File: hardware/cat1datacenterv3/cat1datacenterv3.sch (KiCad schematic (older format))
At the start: 67 parts, among them J1 CAT1UART, J2 USB_C_Receptacle_USB2.0, J3 SPK, J4 IIC, J5 UART1, J6 UART3, J7 SPI, J8 Conn_02x02_Counter_Clockwise, J9 HLK_TTL, U1 Air724, U2 ETA8113, U3 AMS1117-3.3, U4 HLK_7628N

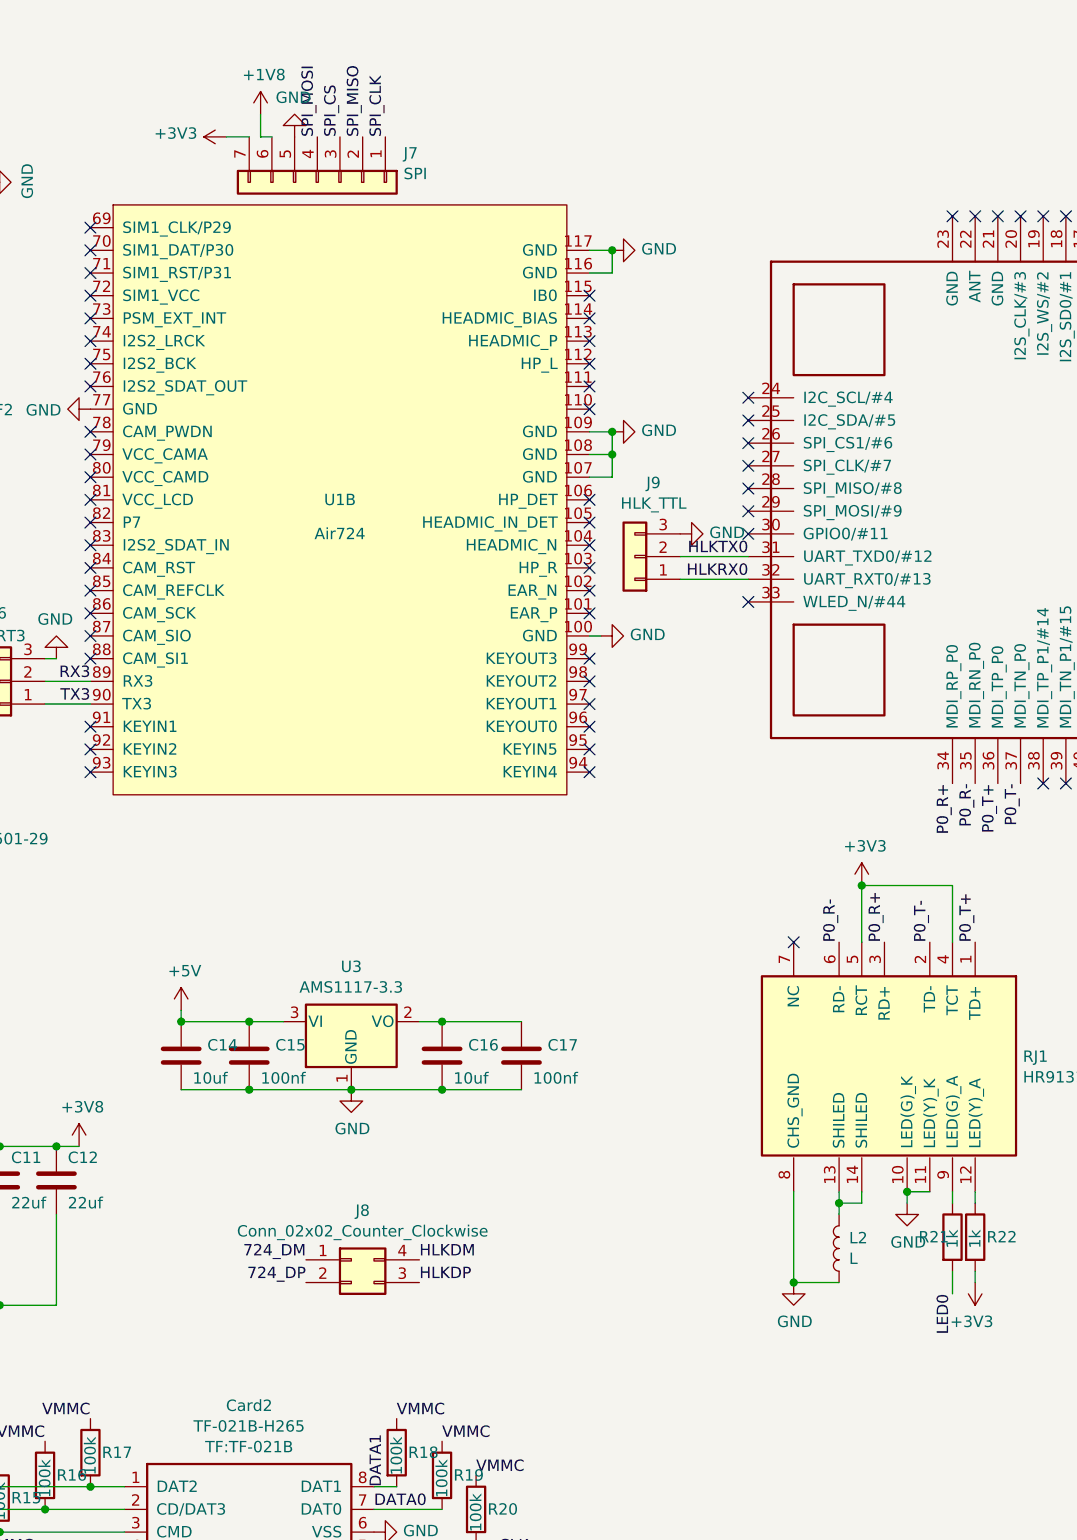
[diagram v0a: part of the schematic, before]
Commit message: add: sim加个srv05
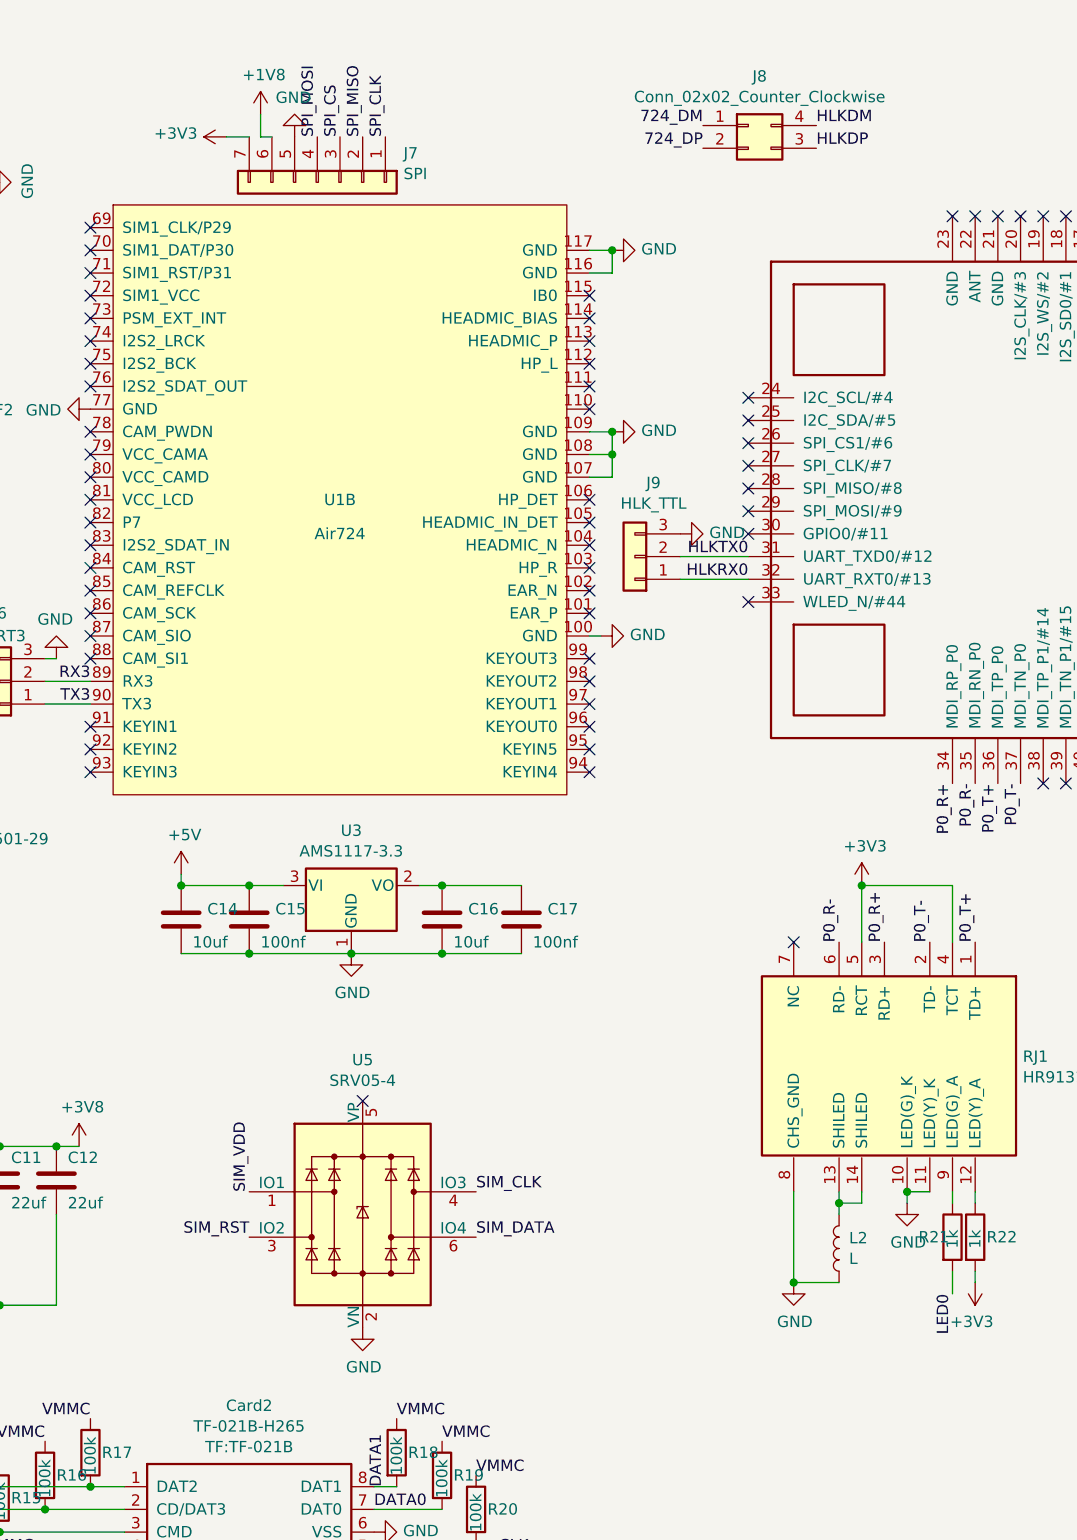
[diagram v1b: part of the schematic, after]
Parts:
- added U5: SRV05-4, Package_TO_SOT_SMD:SOT-23-6, symbol Power_Protection:SRV05-4
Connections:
- net GND: now also U5.2 (VN)
- net SIM_CLK: now also U5.4 (IO3)
- net SIM_DATA: now also U5.6 (IO4)
- net SIM_RST: now also U5.3 (IO2)
- net SIM_VDD: now also U5.1 (IO1)
- no-connect marks 97 -> 98
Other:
- moved on the sheet: C14, C15, C16, C17, J8, U3
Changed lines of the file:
@@
 L Regulator_Linear:AMS1117-3.3 U3
 U 1 1 60BE7D12
-P 6100 4850
-F 0 "U3" H 6100 5092 50  0000 C CNN
-F 1 "AMS1117-3.3" H 6100 5001 50  0000 C CNN
-F 2 "Package_TO_SOT_SMD:SOT-89-3_Handsoldering" H 6100 5050 50  0001 C CNN
-F 3 "http://www.advanced-monolithic.com/pdf/ds1117.pdf" H 6200 4600 50  0001 C CNN
-	1    6100 4850
+P 6100 4250
+F 0 "U3" H 6100 4492 50  0000 C CNN
+F 1 "AMS1117-3.3" H 6100 4401 50  0000 C CNN
+F 2 "Package_TO_SOT_SMD:SOT-89-3_Handsoldering" H 6100 4450 50  0001 C CNN
+F 3 "http://www.advanced-monolithic.com/pdf/ds1117.pdf" H 6200 4000 50  0001 C CNN
+	1    6100 4250
 	1    0    0    -1
 $EndComp
@@
 L Device:C C16
 U 1 1 60C07B48
-P 6500 5000
-F 0 "C16" H 6615 5046 50  0000 L CNN
-F 1 "10uf" H 6550 4900 50  0000 L CNN
-F 2 "Capacitor_SMD:C_0603_1608Metric_Pad1.05x0.95mm_HandSolder" H 6538 4850 50  0001 C CNN
-F 3 "~" H 6500 5000 50  0001 C CNN
-	1    6500 5000
+P 6500 4400
+F 0 "C16" H 6615 4446 50  0000 L CNN
+F 1 "10uf" H 6550 4300 50  0000 L CNN
+F 2 "Capacitor_SMD:C_0603_1608Metric_Pad1.05x0.95mm_HandSolder" H 6538 4250 50  0001 C CNN
+F 3 "~" H 6500 4400 50  0001 C CNN
+	1    6500 4400
 	1    0    0    -1
 $EndComp
@@
 L Device:C C17
 U 1 1 60C088A8
-P 6850 5000
-F 0 "C17" H 6965 5046 50  0000 L CNN
-F 1 "100nf" H 6900 4900 50  0000 L CNN
-F 2 "Capacitor_SMD:C_0603_1608Metric_Pad1.05x0.95mm_HandSolder" H 6888 4850 50  0001 C CNN
-F 3 "~" H 6850 5000 50  0001 C CNN
-	1    6850 5000
-	1    0    0    -1
-$EndComp
-Wire Wire Line
-	6400 4850 6500 4850
-Connection ~ 6500 4850
-Wire Wire Line
-	6500 4850 6850 4850
-Wire Wire Line
-	6100 5150 6500 5150
-Connection ~ 6500 5150
-Wire Wire Line
-	6500 5150 6850 5150
+P 6850 4400
+F 0 "C17" H 6965 4446 50  0000 L CNN
+F 1 "100nf" H 6900 4300 50  0000 L CNN
+F 2 "Capacitor_SMD:C_0603_1608Metric_Pad1.05x0.95mm_HandSolder" H 6888 4250 50  0001 C CNN
+F 3 "~" H 6850 4400 50  0001 C CNN
+	1    6850 4400
+	1    0    0    -1
+$EndComp
+Wire Wire Line
+	6400 4250 6500 4250
+Connection ~ 6500 4250
+Wire Wire Line
+	6500 4250 6850 4250
+Wire Wire Line
+	6100 4550 6500 4550
+Connection ~ 6500 4550
+Wire Wire Line
+	6500 4550 6850 4550
 $Comp
 L power:+5V #PWR043
 U 1 1 60C0F1F9
-P 5350 4800
-F 0 "#PWR043" H 5350 4650 50  0001 C CNN
-F 1 "+5V" H 5365 4973 50  0000 C CNN
-F 2 "" H 5350 4800 50  0001 C CNN
-F 3 "" H 5350 4800 50  0001 C CNN
-	1    5350 4800
+P 5350 4200
+F 0 "#PWR043" H 5350 4050 50  0001 C CNN
+F 1 "+5V" H 5365 4373 50  0000 C CNN
+F 2 "" H 5350 4200 50  0001 C CNN
+F 3 "" H 5350 4200 50  0001 C CNN
+	1    5350 4200
 	1    0    0    -1
 $EndComp
@@
 L Device:C C14
 U 1 1 60C12846
-P 5350 5000
-F 0 "C14" H 5465 5046 50  0000 L CNN
-F 1 "10uf" H 5400 4900 50  0000 L CNN
-F 2 "Capacitor_SMD:C_0603_1608Metric_Pad1.05x0.95mm_HandSolder" H 5388 4850 50  0001 C CNN
-F 3 "~" H 5350 5000 50  0001 C CNN
-	1    5350 5000
+P 5350 4400
+F 0 "C14" H 5465 4446 50  0000 L CNN
+F 1 "10uf" H 5400 4300 50  0000 L CNN
+F 2 "Capacitor_SMD:C_0603_1608Metric_Pad1.05x0.95mm_HandSolder" H 5388 4250 50  0001 C CNN
+F 3 "~" H 5350 4400 50  0001 C CNN
+	1    5350 4400
 	1    0    0    -1
 $EndComp
@@
 L Device:C C15
 U 1 1 60C135CF
-P 5650 5000
-F 0 "C15" H 5765 5046 50  0000 L CNN
-F 1 "100nf" H 5700 4900 50  0000 L CNN
-F 2 "Capacitor_SMD:C_0603_1608Metric_Pad1.05x0.95mm_HandSolder" H 5688 4850 50  0001 C CNN
-F 3 "~" H 5650 5000 50  0001 C CNN
-	1    5650 5000
-	1    0    0    -1
-$EndComp
-Connection ~ 5650 4850
-Wire Wire Line
-	5650 4850 5800 4850
-Wire Wire Line
-	5350 4850 5650 4850
-Wire Wire Line
-	5350 4800 5350 4850
-Connection ~ 5350 4850
-Wire Wire Line
-	5350 5150 5650 5150
-Connection ~ 6100 5150
-Connection ~ 5650 5150
-Wire Wire Line
-	5650 5150 6100 5150
+P 5650 4400
+F 0 "C15" H 5765 4446 50  0000 L CNN
+F 1 "100nf" H 5700 4300 50  0000 L CNN
+F 2 "Capacitor_SMD:C_0603_1608Metric_Pad1.05x0.95mm_HandSolder" H 5688 4250 50  0001 C CNN
+F 3 "~" H 5650 4400 50  0001 C CNN
+	1    5650 4400
+	1    0    0    -1
+$EndComp
+Connection ~ 5650 4250
+Wire Wire Line
+	5650 4250 5800 4250
+Wire Wire Line
+	5350 4250 5650 4250
+Wire Wire Line
+	5350 4200 5350 4250
+Connection ~ 5350 4250
+Wire Wire Line
+	5350 4550 5650 4550
+Connection ~ 6100 4550
+Connection ~ 5650 4550
+Wire Wire Line
+	5650 4550 6100 4550
 $Comp
 L power:GND #PWR047
 U 1 1 60C1F032
-P 6100 5150
-F 0 "#PWR047" H 6100 4900 50  0001 C CNN
-F 1 "GND" H 6105 4977 50  0000 C CNN
-F 2 "" H 6100 5150 50  0001 C CNN
-F 3 "" H 6100 5150 50  0001 C CNN
-	1    6100 5150
+P 6100 4550
+F 0 "#PWR047" H 6100 4300 50  0001 C CNN
+F 1 "GND" H 6105 4377 50  0000 C CNN
+F 2 "" H 6100 4550 50  0001 C CNN
+F 3 "" H 6100 4550 50  0001 C CNN
+	1    6100 4550
 	1    0    0    -1
 $EndComp
@@
 L Connector_Generic:Conn_02x02_Counter_Clockwise J8
 U 1 1 60C45C96
-P 6100 5900
-F 0 "J8" H 6150 6117 50  0000 C CNN
-F 1 "Conn_02x02_Counter_Clockwise" H 6150 6026 50  0000 C CNN
-F 2 "Connector_PinHeader_2.54mm:PinHeader_2x02_P2.54mm_Vertical" H 6100 5900 50  0001 C CNN
-F 3 "~" H 6100 5900 50  0001 C CNN
-	1    6100 5900
-	1    0    0    -1
-$EndComp
-Text Label 5900 5900 2    50   ~ 0
+P 7850 900
+F 0 "J8" H 7900 1117 50  0000 C CNN
+F 1 "Conn_02x02_Counter_Clockwise" H 7900 1026 50  0000 C CNN
+F 2 "Connector_PinHeader_2.54mm:PinHeader_2x02_P2.54mm_Vertical" H 7850 900 50  0001 C CNN
+F 3 "~" H 7850 900 50  0001 C CNN
+	1    7850 900
+	1    0    0    -1
+$EndComp
+Text Label 7650 900  2    50   ~ 0
 724_DM
-Text Label 5900 6000 2    50   ~ 0
+Text Label 7650 1000 2    50   ~ 0
 724_DP
-Text Label 6400 5900 0    50   ~ 0
+Text Label 8150 900  0    50   ~ 0
 HLKDM
-Text Label 6400 6000 0    50   ~ 0
+Text Label 8150 1000 0    50   ~ 0
 HLKDP
 $Comp
@@
 	4500 1150 4450 1150
 Connection ~ 4450 1150
+$Comp
+L Power_Protection:SRV05-4 U5
+U 1 1 60CFB5A0
+P 6150 5700
+F 0 "U5" H 6150 6381 50  0000 C CNN
+F 1 "SRV05-4" H 6150 6290 50  0000 C CNN
+F 2 "Package_TO_SOT_SMD:SOT-23-6" H 6850 5250 50  0001 C CNN
+F 3 "http://www.onsemi.com/pub/Collateral/SRV05-4-D.PDF" H 6150 5700 50  0001 C CNN
+	1    6150 5700
+	1    0    0    -1
+$EndComp
+NoConn ~ 6150 5200
+Text Label 6650 5600 0    50   ~ 0
+SIM_CLK
+Text Label 5650 5800 2    50   ~ 0
+SIM_RST
+Text Label 5650 5600 1    50   ~ 0
+SIM_VDD
+Text Label 6650 5800 0    50   ~ 0
+SIM_DATA
+$Comp
+L power:GND #PWR067
+U 1 1 60D2FD5D
+P 6150 6200
+F 0 "#PWR067" H 6150 5950 50  0001 C CNN
+F 1 "GND" H 6155 6027 50  0000 C CNN
+F 2 "" H 6150 6200 50  0001 C CNN
+F 3 "" H 6150 6200 50  0001 C CNN
+	1    6150 6200
+	1    0    0    -1
+$EndComp
 $EndSCHEMATC
